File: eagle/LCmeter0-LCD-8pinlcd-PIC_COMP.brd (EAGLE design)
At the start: 34 parts, among them IC1 PIC16F876A-X/SP-COMP-B-A, J1 HD44780-4BIT-8PIN, J2 PIC-UART, J3 PIC-ICSPICSP, K2 DS2Y, Q1 20MHz, T1 BC547CBE-A, X1 FREQ, X2 L/C

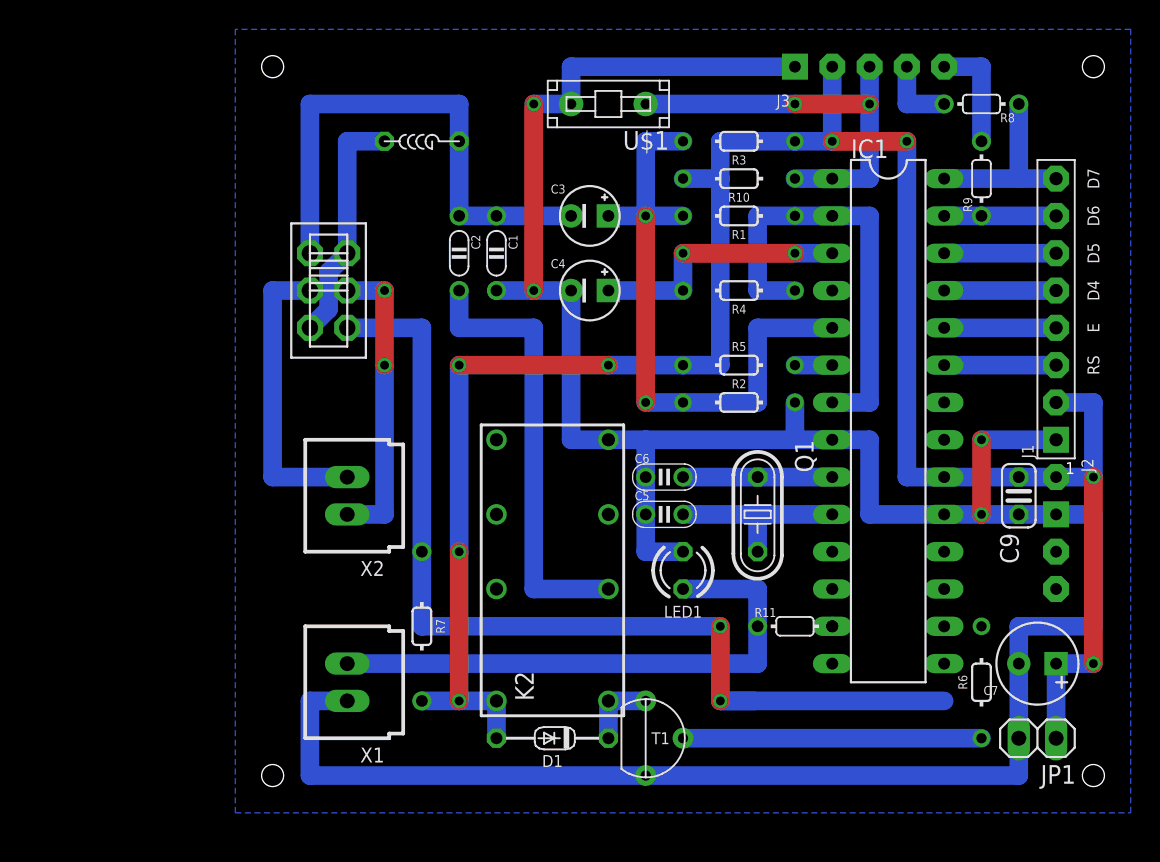
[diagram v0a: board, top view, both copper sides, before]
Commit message: ...
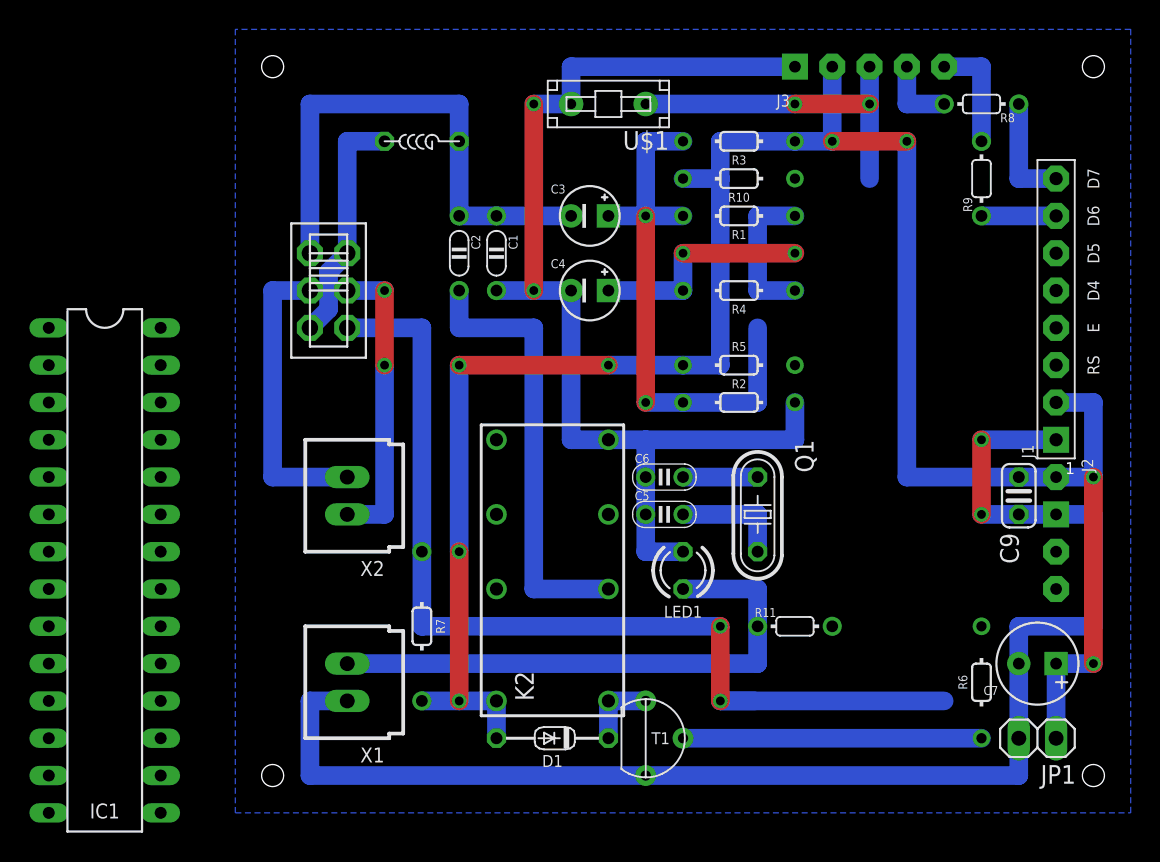
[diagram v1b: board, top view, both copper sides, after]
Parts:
- IC1: value PIC16F876A-X/SP-COMP-B-A -> PIC16F876A-X/SP-COMP-B-A/V; device mcu:DIL28-3 -> mcu:DIL28-3/V
- moved IC1 54.3 mm to (-11.4, 14.0), turned to 0 degrees
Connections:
- net FREQ: now also IC1.11, R11.2
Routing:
- net A0: track 30.5 -> 10.2 mm
- net GND: track 190.5 -> 172.7 mm
- net RS: track 7.62 -> 0.00 mm
- net E: track 7.62 -> 0.00 mm
- net D5: track 7.62 -> 0.00 mm
- net D4: track 7.62 -> 0.00 mm
- net OSC2: track 12.7 -> 7.62 mm
- net OSC1: track 10.2 -> 5.08 mm
- net D7: track 12.7 -> 7.62 mm
- net A3: track 43.2 -> 38.1 mm
- net /MCLR: track 27.9 -> 22.9 mm
- net D6: track 7.62 -> 5.08 mm
- net A4: track 2.54 -> 0.00 mm
- net A1: track 17.8 -> 15.2 mm
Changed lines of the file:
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@@
 <element name="J2" library="pinconn" package="PIC-UART" value="PIC-UART" x="54.61" y="11.43" rot="R90"/>
 <element name="U$1" library="sw" package="PB-1P1T" value="PB-1P-1T" x="22.86" y="45.72" rot="R180"/>
-<element name="IC1" library="mcu" package="DIL28-3" value="PIC16F876A-X/SP-COMP-B-A" x="41.91" y="24.13" smashed="yes" rot="R270">
-<attribute name="NAME" x="39.37" y="42.037" size="1.27" layer="25"/>
-<attribute name="VALUE" x="41.2877" y="33.8455" size="1.016" layer="27" rot="R270"/>
-</element>
+<element name="IC1" library="mcu" package="DIL28-3/V" value="PIC16F876A-X/SP-COMP-B-A/V" x="-11.43" y="13.97"/>
 </elements>
 <signals>
@@
 <wire x1="25.4" y1="38.1" x2="22.86" y2="38.1" width="1.27" layer="16"/>
 <contactref element="IC1" pad="5"/>
-<wire x1="38.1" y1="30.48" x2="33.02" y2="30.48" width="1.27" layer="16"/>
+<wire x1="-15.24" y1="20.32" x2="25.4" y2="25.4" width="0" layer="19" extent="16-16"/>
 </signal>
 <signal name="N$2">
@@
 <contactref element="IC1" pad="2"/>
 <contactref element="IC1" pad="7"/>
-<wire x1="38.1" y1="38.1" x2="35.56" y2="38.1" width="1.27" layer="16"/>
-<wire x1="38.1" y1="25.4" x2="40.64" y2="25.4" width="1.27" layer="16"/>
-<wire x1="40.64" y1="25.4" x2="40.64" y2="38.1" width="1.27" layer="16"/>
-<wire x1="40.64" y1="38.1" x2="38.1" y2="38.1" width="1.27" layer="16"/>
+<wire x1="-15.24" y1="27.94" x2="33.02" y2="33.02" width="0" layer="19" extent="16-16"/>
+<wire x1="-15.24" y1="15.24" x2="-15.24" y2="27.94" width="0" layer="19" extent="1-1"/>
 </signal>
 <signal name="A1">
@@
 <wire x1="27.94" y1="35.56" x2="27.94" y2="33.02" width="1.27" layer="16"/>
 <contactref element="IC1" pad="3"/>
-<wire x1="35.56" y1="35.56" x2="38.1" y2="35.56" width="1.27" layer="16"/>
+<wire x1="-15.24" y1="25.4" x2="22.86" y2="33.02" width="0" layer="19" extent="1-1"/>
 </signal>
 <signal name="GND">
@@
 <via x="17.78" y="45.72" extent="1-16" drill="0.6" shape="square"/>
 <wire x1="17.78" y1="45.72" x2="17.78" y2="33.02" width="1.27" layer="1"/>
-<contactref element="IC1" pad="19"/>
-<contactref element="IC1" pad="8"/>
-<wire x1="35.56" y1="22.86" x2="38.1" y2="22.86" width="1.27" layer="16"/>
-<wire x1="38.1" y1="22.86" x2="40.64" y2="22.86" width="1.27" layer="16"/>
-<wire x1="40.64" y1="22.86" x2="40.64" y2="17.78" width="1.27" layer="16"/>
-<wire x1="40.64" y1="17.78" x2="45.72" y2="17.78" width="1.27" layer="16"/>
-<wire x1="48.26" y1="17.78" x2="45.72" y2="17.78" width="1.27" layer="16"/>
 <polygon width="0.254" layer="16" isolate="1.27">
 <vertex x="-2.54" y="50.8"/>
@@
 <vertex x="58.42" y="50.8"/>
 </polygon>
+<contactref element="IC1" pad="19"/>
+<contactref element="IC1" pad="8"/>
+<wire x1="-7.62" y1="7.62" x2="-15.24" y2="12.7" width="0" layer="19" extent="1-1"/>
+<wire x1="2.54" y1="5.08" x2="-7.62" y2="7.62" width="0" layer="19" extent="16-16"/>
 </signal>
 <signal name="N$7">
@@
 <wire x1="27.94" y1="20.32" x2="33.02" y2="20.32" width="1.27" layer="16"/>
 <contactref element="IC1" pad="9"/>
-<wire x1="33.02" y1="20.32" x2="38.1" y2="20.32" width="1.27" layer="16"/>
+<wire x1="-15.24" y1="10.16" x2="27.94" y2="20.32" width="0" layer="19" extent="1-1"/>
 </signal>
 <signal name="OSC2">
@@
 <wire x1="33.02" y1="17.78" x2="27.94" y2="17.78" width="1.27" layer="16"/>
 <contactref element="IC1" pad="10"/>
-<wire x1="38.1" y1="17.78" x2="33.02" y2="17.78" width="1.27" layer="16"/>
+<wire x1="-15.24" y1="7.62" x2="27.94" y2="17.78" width="0" layer="19" extent="1-1"/>
 </signal>
 <signal name="VCC">
@@
 <contactref element="J1" pad="5"/>
 <contactref element="IC1" pad="25"/>
-<wire x1="45.72" y1="33.02" x2="53.34" y2="33.02" width="1.27" layer="16"/>
+<wire x1="-7.62" y1="22.86" x2="53.34" y2="33.02" width="0" layer="19" extent="1-1"/>
 </signal>
 <signal name="E">
 <contactref element="J1" pad="4"/>
 <contactref element="IC1" pad="24"/>
-<wire x1="53.34" y1="30.48" x2="45.72" y2="30.48" width="1.27" layer="16"/>
+<wire x1="-7.62" y1="20.32" x2="53.34" y2="30.48" width="0" layer="19" extent="1-1"/>
 </signal>
 <signal name="RS">
 <contactref element="J1" pad="3"/>
 <contactref element="IC1" pad="23"/>
-<wire x1="45.72" y1="27.94" x2="53.34" y2="27.94" width="1.27" layer="16"/>
+<wire x1="-7.62" y1="17.78" x2="53.34" y2="27.94" width="0" layer="19" extent="1-1"/>
 </signal>
 <signal name="A4">
 <contactref element="R5" pad="2"/>
 <contactref element="IC1" pad="6"/>
-<wire x1="35.56" y1="27.94" x2="38.1" y2="27.94" width="1.27" layer="16"/>
+<wire x1="-15.24" y1="17.78" x2="35.56" y2="27.94" width="0" layer="19" extent="1-1"/>
 </signal>
 <signal name="/LC">
@@
 <wire x1="35.56" y1="45.72" x2="25.4" y2="45.72" width="1.27" layer="16"/>
 <contactref element="IC1" pad="1"/>
-<wire x1="38.1" y1="40.64" x2="40.64" y2="40.64" width="1.27" layer="16"/>
-<wire x1="38.1" y1="40.64" x2="35.56" y2="40.64" width="1.27" layer="16"/>
+<wire x1="40.64" y1="40.64" x2="35.56" y2="40.64" width="0" layer="19" extent="16-16"/>
+<wire x1="-15.24" y1="30.48" x2="25.4" y2="45.72" width="0" layer="19" extent="1-1"/>
 </signal>
 <signal name="RC5">
@@
 <contactref element="J1" pad="6"/>
 <contactref element="IC1" pad="26"/>
-<wire x1="53.34" y1="35.56" x2="45.72" y2="35.56" width="1.27" layer="16"/>
+<wire x1="-7.62" y1="25.4" x2="53.34" y2="35.56" width="0" layer="19" extent="1-1"/>
 </signal>
 <signal name="D6">
@@
 <wire x1="48.26" y1="38.1" x2="53.34" y2="38.1" width="1.27" layer="16"/>
 <contactref element="IC1" pad="27"/>
-<wire x1="45.72" y1="38.1" x2="48.26" y2="38.1" width="1.27" layer="16"/>
+<wire x1="-7.62" y1="27.94" x2="48.26" y2="38.1" width="0" layer="19" extent="1-1"/>
 </signal>
 <signal name="D7">
@@
 <wire x1="53.34" y1="40.64" x2="50.8" y2="40.64" width="1.27" layer="16"/>
 <contactref element="IC1" pad="28"/>
-<wire x1="45.72" y1="40.64" x2="50.8" y2="40.64" width="1.27" layer="16"/>
+<wire x1="-7.62" y1="30.48" x2="50.8" y2="40.64" width="0" layer="19" extent="16-16"/>
 </signal>
 <signal name="C2_CON">
@@
 <wire x1="5.08" y1="7.62" x2="33.02" y2="7.62" width="1.27" layer="16"/>
 <wire x1="33.02" y1="7.62" x2="33.02" y2="10.16" width="1.27" layer="16"/>
+<contactref element="IC1" pad="11"/>
+<contactref element="R11" pad="2"/>
+<wire x1="33.02" y1="10.16" x2="38.1" y2="10.16" width="0" layer="19" extent="16-16"/>
+<wire x1="-15.24" y1="5.08" x2="5.08" y2="7.62" width="0" layer="19" extent="1-1"/>
 </signal>
 <signal name="N$1">
